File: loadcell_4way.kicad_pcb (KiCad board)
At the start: 2 copper layers, 140 x 60 mm, 115 parts, among them J1 USB_B_Micro, J10 Conn_01x05, J2 Battery, J3 OLDED_Screen, J4 Conn_01x05, J5 Conn_01x05, J6 Conn_01x05, Q1 FDS6892A, Q2 BSS138, Q3 SM2331PSA P-MOSFET, Q5 BSS138, Q7 BSS138, Q8 BSS138, SW1 SW_Push, SW2 SW_Push, SW3 SW_Push, U1 FS312F-G, U10 ADS1234IPW, U2 MT3608, U3 TP4056, U4 ESP32-C3-WROOM-02, U5 LM1117-3.3, U7 AP2127K-ADJ, U9 CH340C

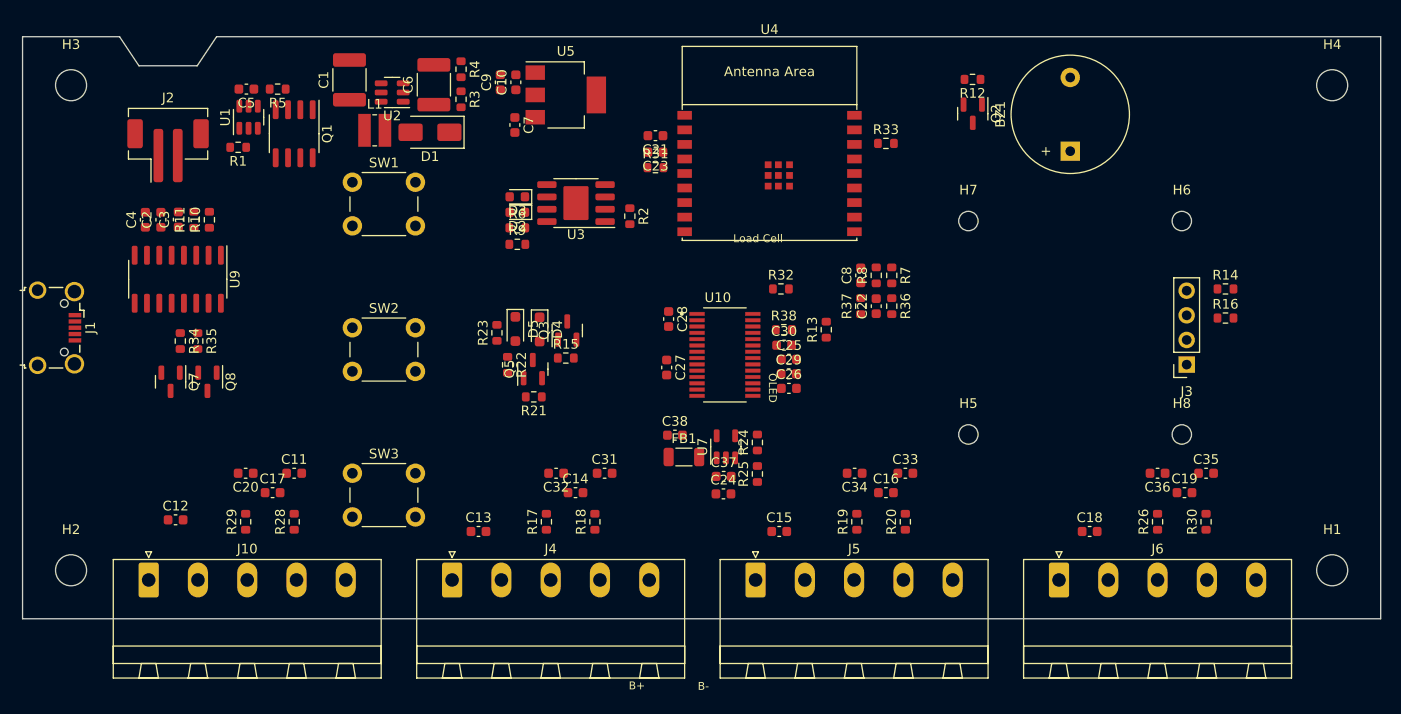
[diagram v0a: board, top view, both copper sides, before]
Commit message: pcb wip
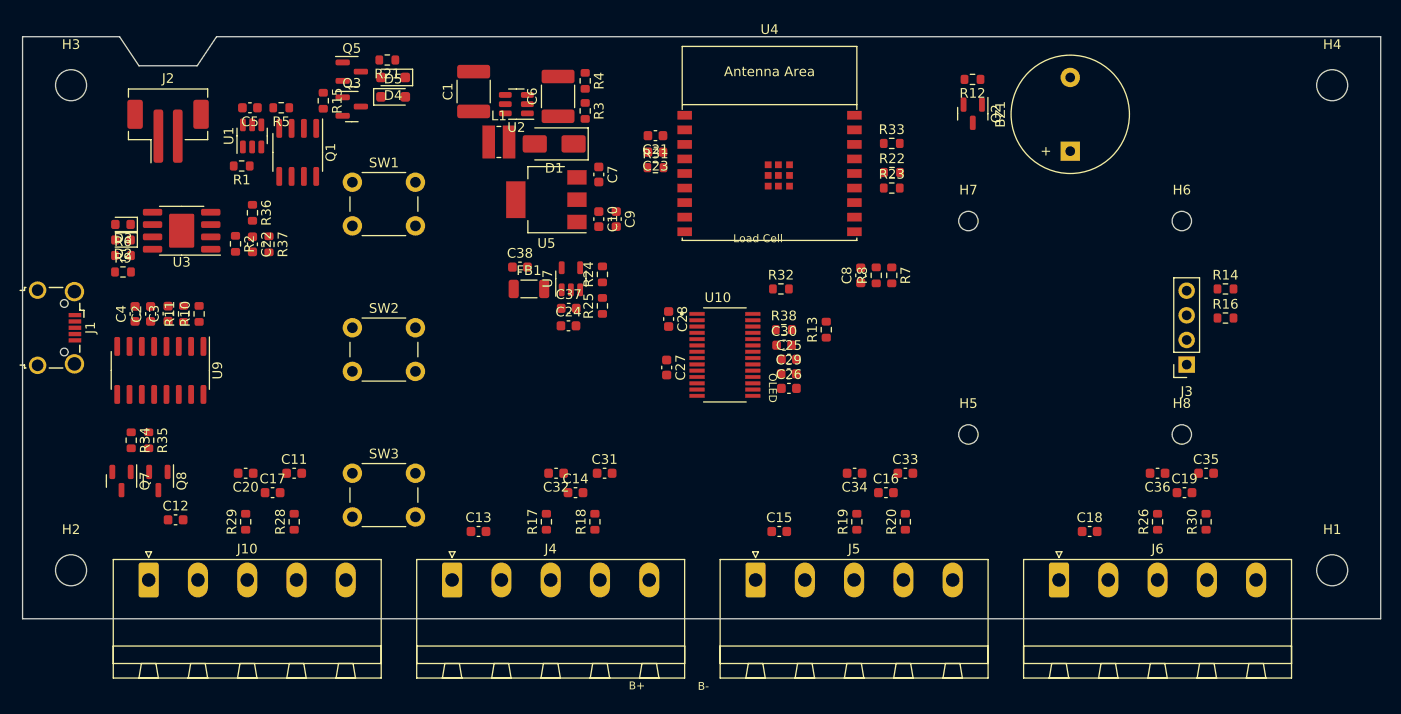
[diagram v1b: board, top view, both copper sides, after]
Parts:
- moved R36 66.6 mm to (123.7, 58.1)
- moved C22 64.6 mm to (123.7, 61.4), turned to -90 degrees
- moved R37 61.3 mm to (125.4, 61.4), turned to -90 degrees
- moved R22 44.3 mm to (189.6, 54.0), turned to 0 degrees
- moved R23 43.4 mm to (189.6, 55.6), turned to 0 degrees
- moved D2 40.7 mm to (110.4, 61.0)
- moved D3 40.7 mm to (110.4, 59.4)
- moved R2 40.7 mm to (122.0, 61.4)
- moved R6 40.7 mm to (110.4, 62.6)
- moved R9 40.7 mm to (110.4, 64.3)
- moved U3 40.7 mm to (116.4, 60.0)
- moved R21 37.9 mm to (137.6, 42.4)
- moved R15 36.4 mm to (131.0, 46.6), turned to -90 degrees
- moved Q5 35.9 mm to (133.9, 43.6), turned to 0 degrees
- moved Q3 32.0 mm to (133.9, 47.2), turned to 0 degrees
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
